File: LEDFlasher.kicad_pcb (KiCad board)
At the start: 2 copper layers, 63.5 x 53.3 mm, 16 parts, among them Q1 2N3904, SW1 SW_Push, T1 Transformer_1P_1S, U1 4001

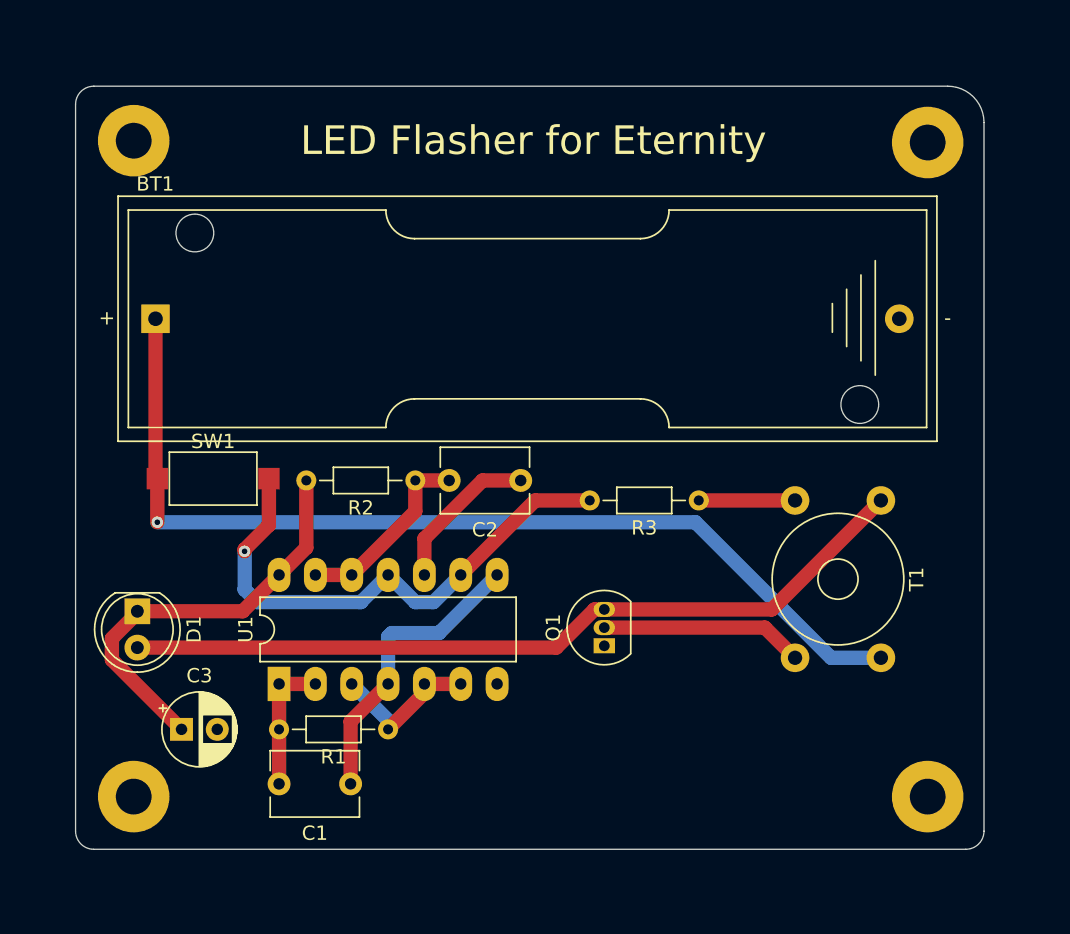
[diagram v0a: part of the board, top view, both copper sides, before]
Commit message: Review changes
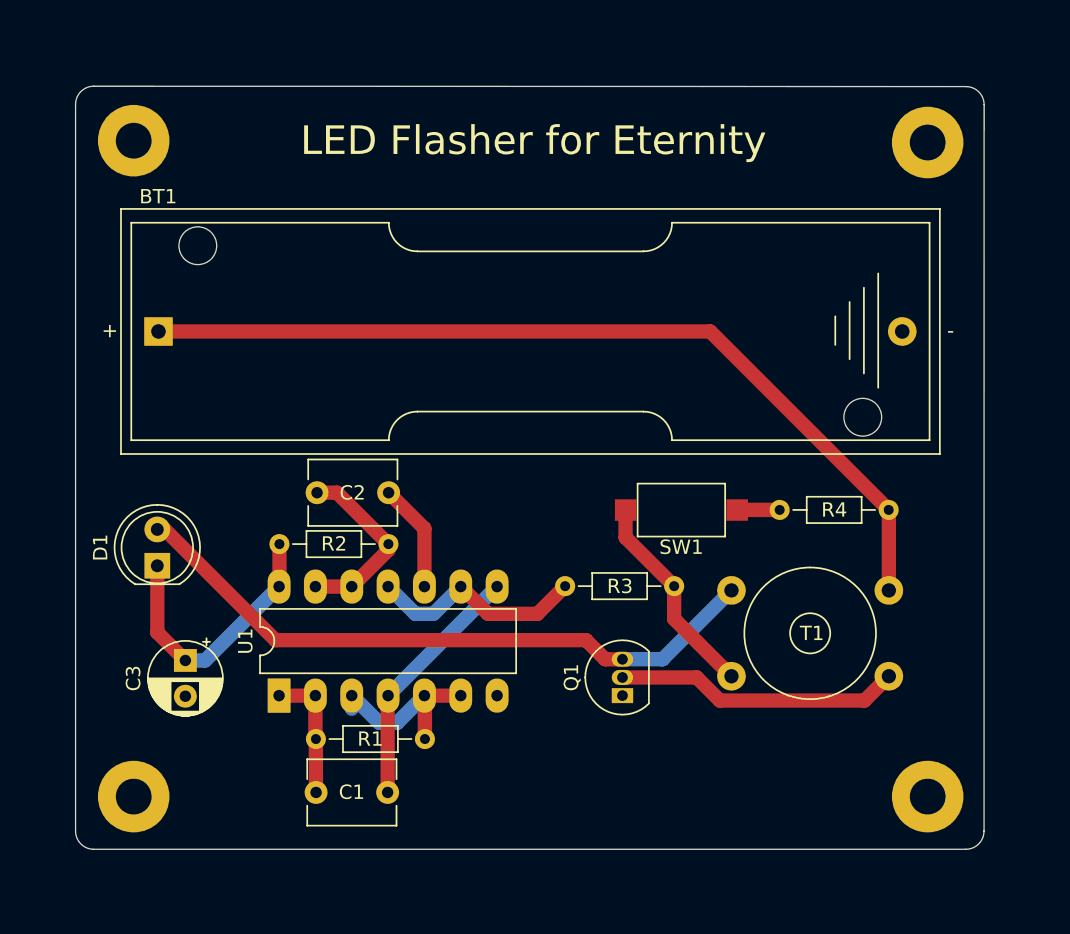
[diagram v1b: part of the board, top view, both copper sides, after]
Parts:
- added R4: 4k7, Resistor_THT:R_Axial_DIN0204_L3.6mm_D1.6mm_P7.62mm_Horizontal, F.Cu at (155.9, 93.2)
- moved SW1 32.8 mm to (141.4, 93.3), turned to 180 degrees
- moved T1 13.1 mm to (144.9, 104.9), turned to 0 degrees
- moved C2 9.27 mm to (120.9, 92.0)
- moved R3 6.23 mm to (140.9, 98.6)
- moved R2 4.83 mm to (120.9, 95.6)
- moved C3 4.82 mm to (106.7, 103.8), turned to 270 degrees
- moved Q1 3.71 mm to (137.3, 106.2)
- moved D1 3.47 mm to (104.8, 97.1), turned to 90 degrees
- moved R1 2.67 mm to (123.5, 109.3)
- moved C1 2.66 mm to (120.9, 113.0)
- moved BT1 0.91 mm to (104.9, 80.8)
- moved U1 0.82 mm to (113.3, 106.2)
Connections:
- SW1 pad 1: Net-(BT1-Pad1) -> Net-(R4-Pad2)
- SW1 pad 2: Net-(R3-Pad2) -> Net-(R3-Pad1)
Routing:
- net Net-(R3-Pad2): track 37.5 -> 15.5 mm, vias 1 -> 0
- net Net-(D1-Pad2): track 56.2 -> 45.9 mm
- net Net-(C3-Pad1): track 29.4 -> 19.1 mm
- net Net-(R3-Pad1): track 6.73 -> 14.7 mm
- net Net-(BT1-Pad1): track 68.8 -> 61.8 mm, vias 1 -> 0
- net Net-(Q1-Pad2): track 14.2 -> 20.0 mm
- net Net-(C2-Pad1): track 11.0 -> 7.60 mm
- net Net-(C1-Pad1): track 20.8 -> 17.6 mm
- net Net-(R4-Pad2): track 0.00 -> 2.98 mm
- net Net-(R1-Pad1): track 11.0 -> 13.2 mm
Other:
- outline, holes or cut-outs redrawn
